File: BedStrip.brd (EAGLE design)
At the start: 72 x 48 mm, 25 parts, among them IC1 74AHCT2G125DP,125, IC4 LM2596S

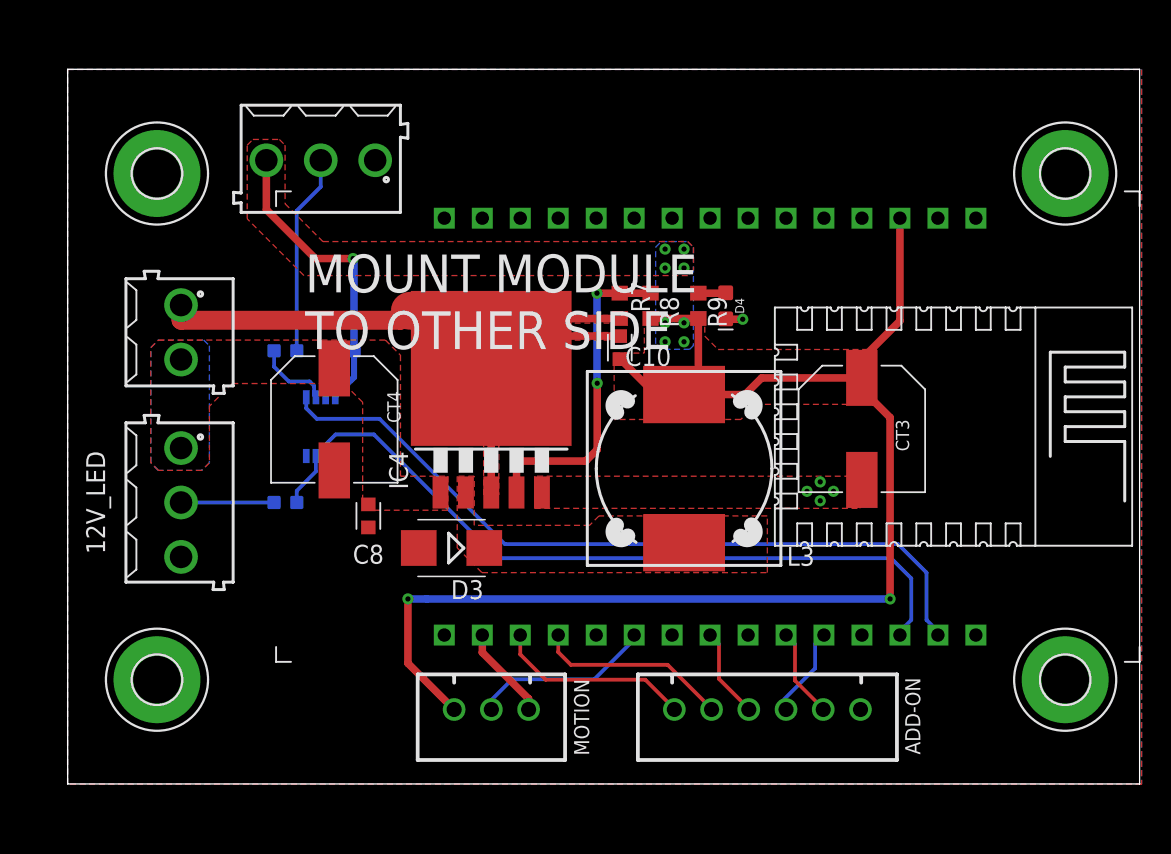
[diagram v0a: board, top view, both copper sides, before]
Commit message: Ready for PCB MFG
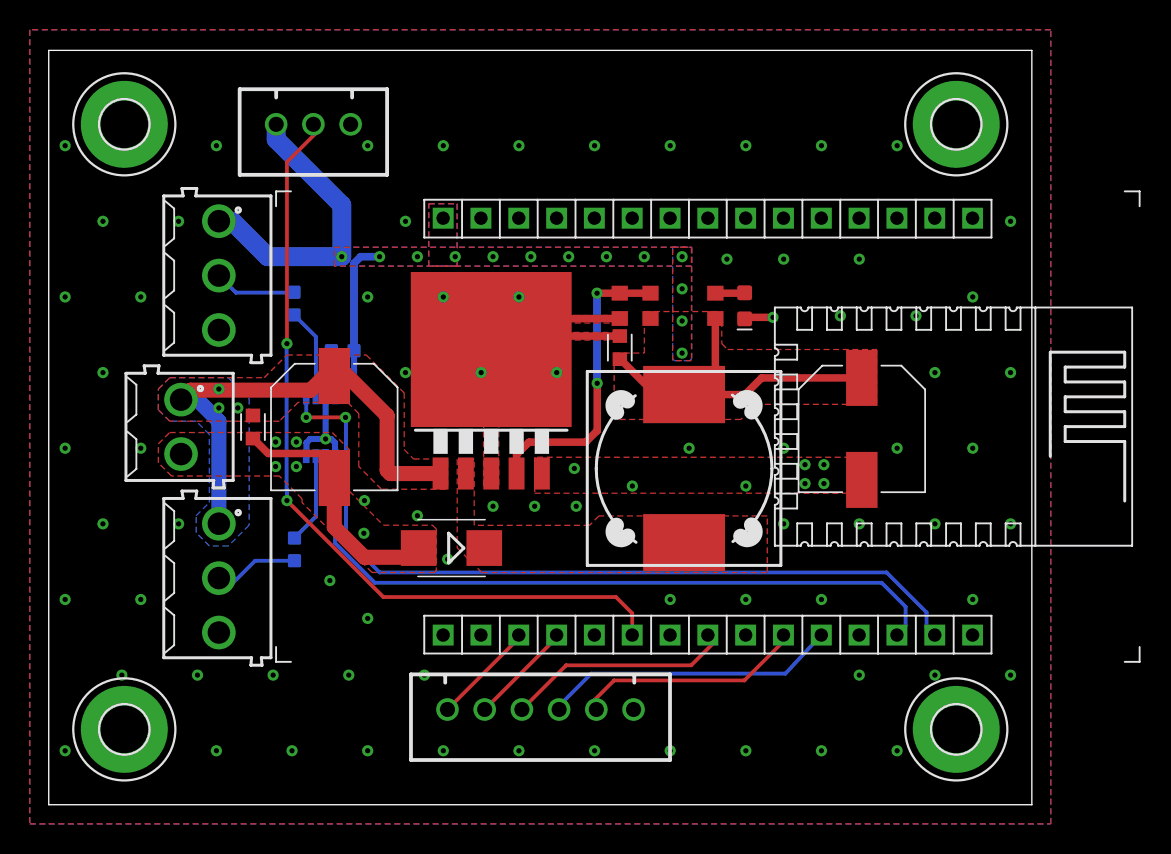
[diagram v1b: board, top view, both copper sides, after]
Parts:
- removed MOTION: JST-XH-03-PIN-VERT-ROUND-PAD, JST XH Connectors:JST-XH-03-VERT-ROUND-PAD
- added PIR.SENSOR: JST-XH-03-PIN-VERT-ROUND-PAD, JST XH Connectors:JST-XH-03-VERT-ROUND-PAD
- moved ADD-ON 15.2 mm to (0.01, -11.4)
- moved 5V_LED 10.3 mm to (-21.6, 17.8), turned to 270 degrees
- moved C8 9.78 mm to (-19.3, 7.61)
- moved H1 8.04 mm to (27.9, -12.7)
- moved H4 8.03 mm to (27.9, 27.9)
- moved POWER 6.35 mm to (-24.1, 7.62)
- moved 12V_LED 5.68 mm to (-21.6, -2.54)
- moved H3 3.99 mm to (-27.9, -12.7)
- moved H2 3.97 mm to (-27.9, 27.9)
- moved R1 3.22 mm to (-16.5, 15.9), turned to 0 degrees
- moved R5 3.21 mm to (-16.5, -0.61), turned to 180 degrees
- moved D4 1.27 mm to (13.7, 15.7)
- moved IC4 1.27 mm to (-3.30, 10.3)
- moved R9 1.14 mm to (11.8, 15.7)
- moved CT4 0.51 mm to (-13.8, 7.61)
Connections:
- net 3.3V renamed VCC_3V3.2
- new net VCC_3V3.1: U$1.3.3V
- new net VCC_3V3.3: U$1.3.3V_3
- net 12V: now also POWER.1; no longer POWER.2
- net 5V: now also 5V_LED.1, PIR.SENSOR.3, U$1.VIN; no longer 5V_LED.3, MOTION.3, U$1.VUSB
- net GND: now also 5V_LED.3, PIR.SENSOR.1, POWER.2; no longer 5V_LED.1, MOTION.1, POWER.1
- net IO13: now also PIR.SENSOR.2; no longer MOTION.2
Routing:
- net 5V: track 116.0 -> 54.2 mm, vias 11 -> 13
- net IO13: track 12.2 -> 53.9 mm, vias 0 -> 2
- net 12V: track 0.00 -> 33.5 mm, vias 0 -> 3
- net GND: track 62.4 -> 47.5 mm, vias 5 -> 90
- net IO2: track 6.27 -> 19.9 mm
- net VCC_3V3.2: track 6.04 -> 15.6 mm
- net IO14: track 6.08 -> 15.3 mm
- net WS2812_DATA: track 13.5 -> 5.53 mm
- net TXD0: track 13.2 -> 7.06 mm
- net RXD0: track 13.1 -> 7.11 mm
- net IO5: track 51.5 -> 55.0 mm, vias 0 -> 2
- net N$12: track 3.65 -> 6.11 mm
- net N$7: track 21.8 -> 20.2 mm
- net N$1: track 5.10 -> 6.14 mm
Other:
- board size 72 x 48 mm -> 66 x 50.7 mm
